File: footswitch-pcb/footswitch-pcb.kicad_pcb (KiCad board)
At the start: 2 copper layers, 60 x 30 mm, 14 parts, among them Q1 BUK7880-55A, U1 SeeeduinoXIAO

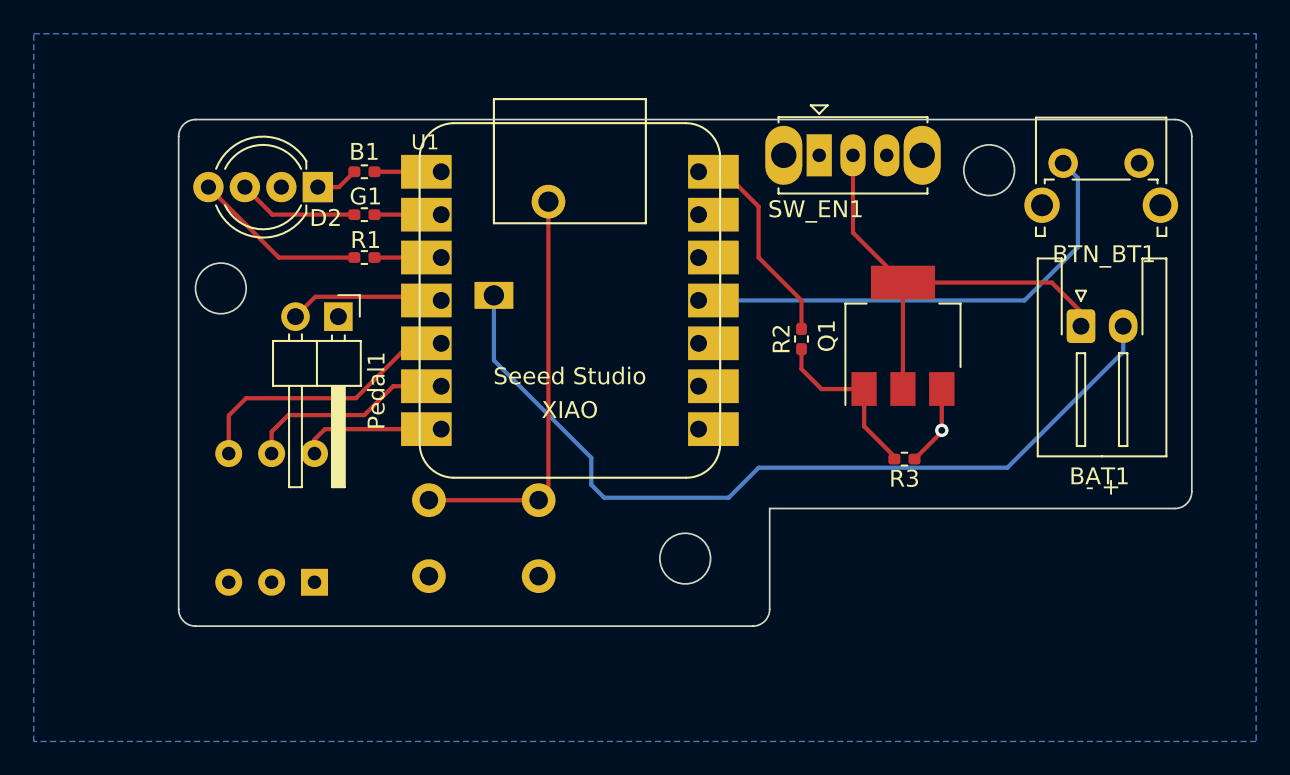
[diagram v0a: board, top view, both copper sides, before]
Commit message: v3
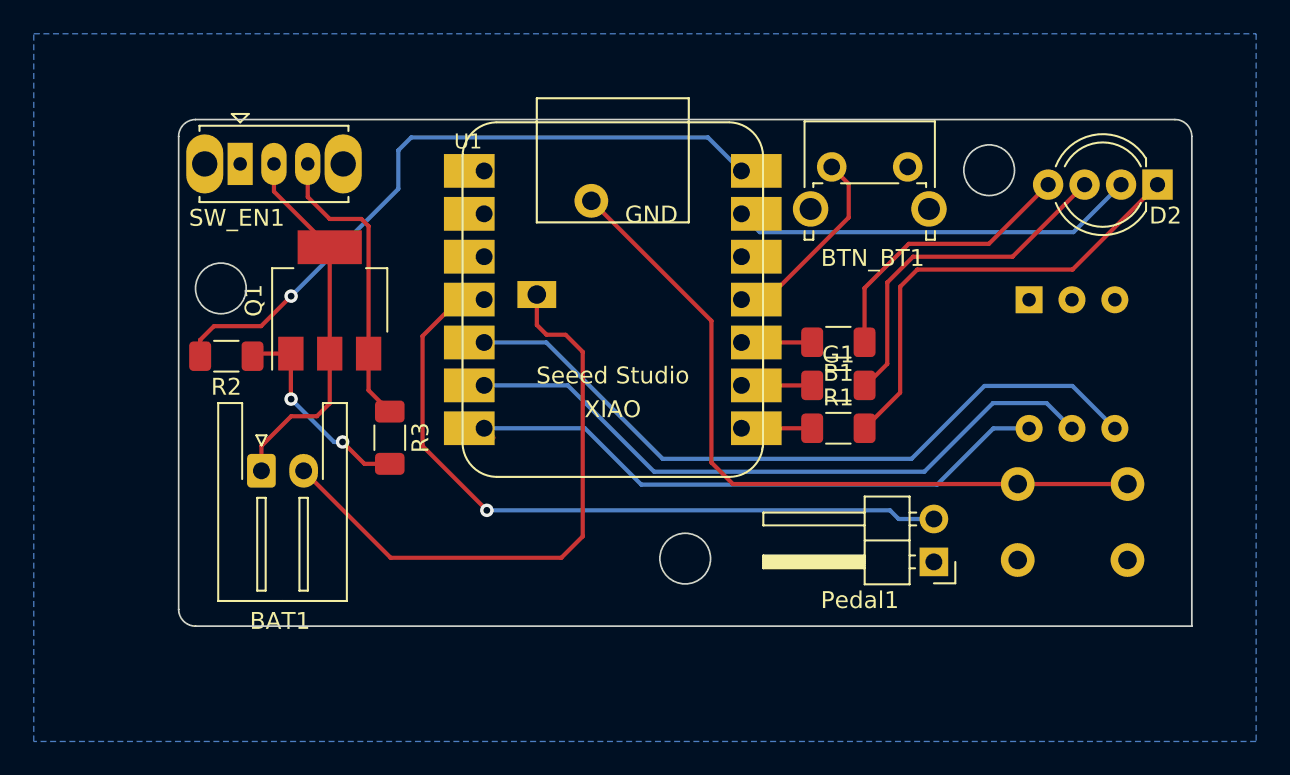
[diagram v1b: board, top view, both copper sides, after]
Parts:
- B1, G1, R1, R2, R3: footprint Resistor_SMD:R_0402_1005Metric_Pad0.72x0.64mm_HandSolder -> Resistor_SMD:R_1206_3216Metric_Pad1.30x1.75mm_HandSolder
- moved D2 49.7 mm to (168.1, 75.0)
- moved BAT1 49.3 mm to (115.1, 91.9)
- moved DIP_MODE1 45.5 mm to (160.5, 81.8), turned to -90 degrees
- moved Pedal1 38.1 mm to (154.9, 97.3), turned to 180 degrees
- moved BTN_RESET1 34.9 mm to (166.4, 92.7)
- moved SW_EN1 34.3 mm to (113.8, 73.7)
- moved R2 34.1 mm to (113.0, 85.1), turned to 180 degrees
- moved Q1 34.0 mm to (119.1, 81.8)
- moved R3 30.5 mm to (122.7, 90.0), turned to -90 degrees
- moved G1 29.8 mm to (149.2, 86.9), turned to 0 degrees
- moved R1 29.8 mm to (149.2, 89.4), turned to 0 degrees
- moved B1 29.8 mm to (149.2, 84.3), turned to 180 degrees
- moved BTN_BT1 13.7 mm to (148.9, 73.9)
- moved U1 2.54 mm to (135.9, 81.8)
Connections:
- B1 pad 2: PIN_LEDR -> PIN_LEDB
- D2 pad 1: Net-(B1-Pad1) -> Net-(D2-Pad1)
- D2 pad 4: Net-(D2-Pad4) -> Net-(B1-Pad1)
- R1 pad 1: PIN_LEDB -> PIN_LEDR
- R1 pad 2: Net-(D2-Pad4) -> Net-(D2-Pad1)
- U1 pad 1: PIN_LEDR -> unconnected-(U1-Pad1)
- U1 pad 10: unconnected-(U1-Pad10) -> PIN_LEDB
- U1 pad 2: PIN_LEDG -> unconnected-(U1-Pad2)
- U1 pad 3: PIN_LEDB -> unconnected-(U1-Pad3)
- U1 pad 8: unconnected-(U1-Pad8) -> PIN_LEDR
- U1 pad 9: unconnected-(U1-Pad9) -> PIN_LEDG
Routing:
- net GND: track 4.82 -> 41.9 mm, vias 1 -> 0
- net PIN_PEDAL: track 9.21 -> 43.1 mm, vias 0 -> 1
- net 5V_USB: track 12.7 -> 40.1 mm, vias 0 -> 1
- net PIN_LAYER3: track 8.59 -> 35.8 mm
- net Net-(D2-Pad1): track 0.00 -> 27.0 mm
- net PIN_LAYER2: track 12.4 -> 39.2 mm
- net PIN_LAYER1: track 16.6 -> 43.0 mm
- net RESET: track 24.4 -> 43.6 mm
- net PIN_BT: track 29.1 -> 11.8 mm
- net BAT+: track 50.5 -> 35.3 mm
- net Net-(B1-Pad1): track 2.54 -> 16.6 mm
- net Net-(D2-Pad3): track 7.16 -> 20.8 mm
- net Net-(D2-Pad4): track 10.4 -> 0.00 mm
- net Net-(BAT1-Pad1): track 27.2 -> 22.1 mm
- net Net-(Q1-Pad1): track 10.3 -> 12.5 mm, vias 0 -> 2
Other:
- outline, holes or cut-outs redrawn
- board text removed: "- +"

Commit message: Possibly final version of PCB?
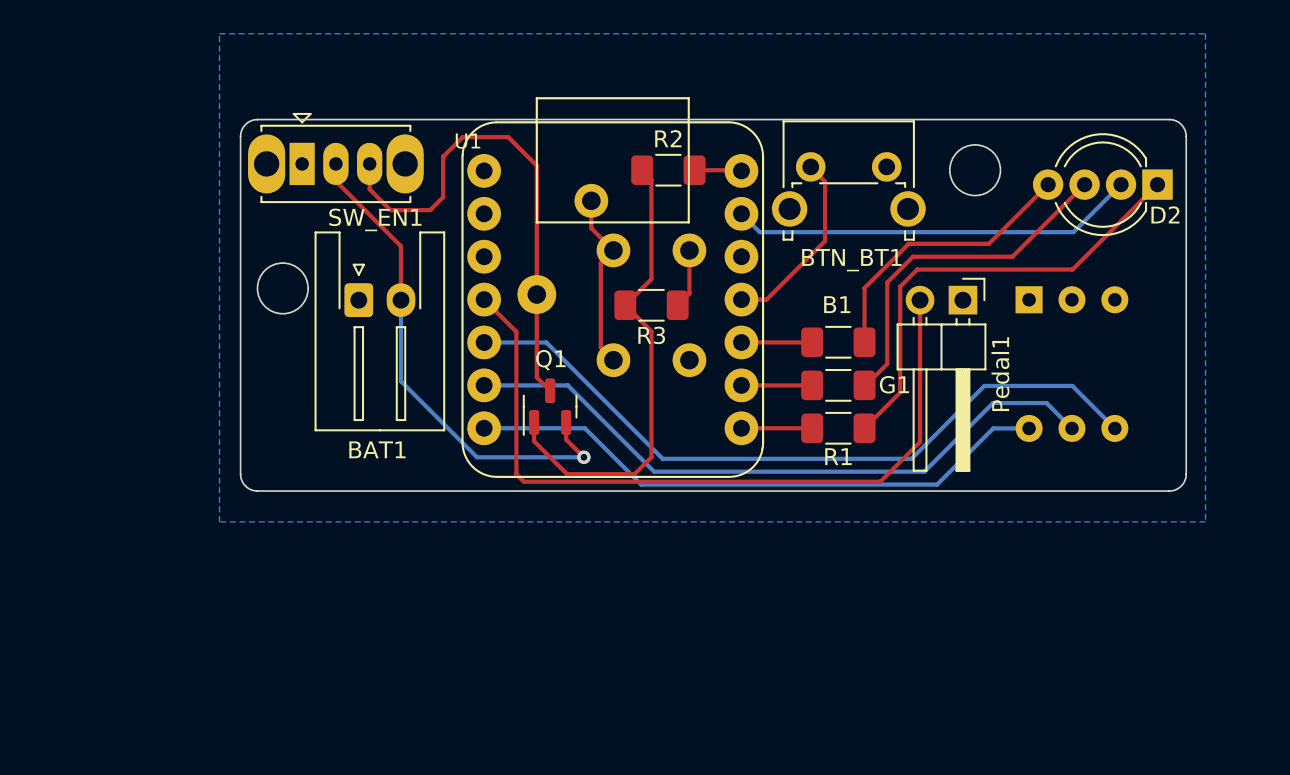
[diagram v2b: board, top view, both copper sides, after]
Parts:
- Q1: footprint Package_TO_SOT_SMD:SOT-223-3_TabPin2 -> Package_TO_SOT_SMD:SOT-23
- moved BTN_RESET1 33.4 mm to (135.9, 78.9), turned to -90 degrees
- moved R2 28.4 mm to (139.2, 74.1), turned to 0 degrees
- moved R3 17.4 mm to (138.2, 82.1), turned to 180 degrees
- moved Pedal1 15.6 mm to (156.6, 81.8), turned to -90 degrees
- moved Q1 14.5 mm to (132.2, 88.1)
- moved BAT1 11.6 mm to (120.8, 81.8)
- moved SW_EN1 3.67 mm to (117.5, 73.7)
- moved BTN_BT1 1.24 mm to (147.6, 73.9)
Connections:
- BAT1 pad 1: Net-(BAT1-Pad1) -> GND
- BAT1 pad 2: BAT+ -> Net-(BAT1-Pad2)
- DIP_MODE1 pad 1: GNDS -> GND
- DIP_MODE1 pad 2: GNDS -> GND
- DIP_MODE1 pad 3: GNDS -> GND
- Q1 pad 2: Net-(BAT1-Pad1) -> Net-(BAT1-Pad2)
- Q1 pad 3: GND -> MCUBAT+
- SW_EN1 pad 2: Net-(BAT1-Pad1) -> Net-(BAT1-Pad2)
- SW_EN1 pad 3: GND -> MCUBAT+
- U1 pad 22: BAT+ -> MCUBAT+
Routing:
- net 5V_USB: track 40.1 -> 2.80 mm, vias 1 -> 0
- net BAT+: track 35.3 -> 0.00 mm
- net RESET: track 43.6 -> 10.6 mm
- net Net-(BAT1-Pad2): track 0.00 -> 29.7 mm, vias 0 -> 1
- net MCUBAT+: track 0.00 -> 29.5 mm
- net Net-(BAT1-Pad1): track 22.1 -> 0.00 mm
- net Net-(Q1-Pad1): track 12.5 -> 27.8 mm, vias 2 -> 0
- net GND: track 41.9 -> 27.6 mm
- net PIN_PEDAL: track 43.1 -> 44.6 mm, vias 1 -> 0
- net PIN_LAYER3: track 35.8 -> 35.0 mm
- net PIN_BT: track 11.8 -> 11.1 mm
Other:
- board size 60 x 30 mm -> 56 x 22 mm
- board text removed: "GND"
